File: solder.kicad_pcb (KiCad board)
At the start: 2 copper layers, 83.3 x 92.9 mm, 22 parts, among them M1 Motor_DC, SW2 SW_Push, SW3 SW_Push, SW4 SW_Push

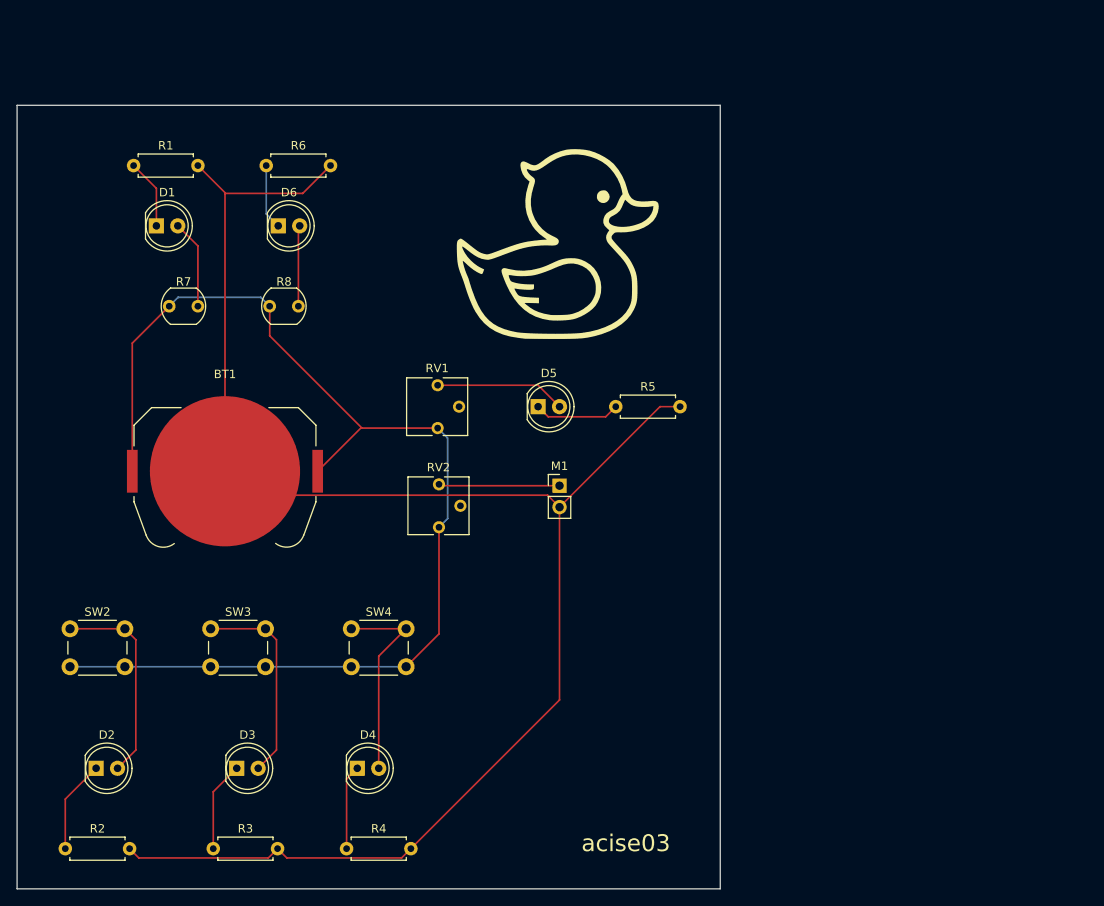
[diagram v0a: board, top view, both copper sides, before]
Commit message: gg
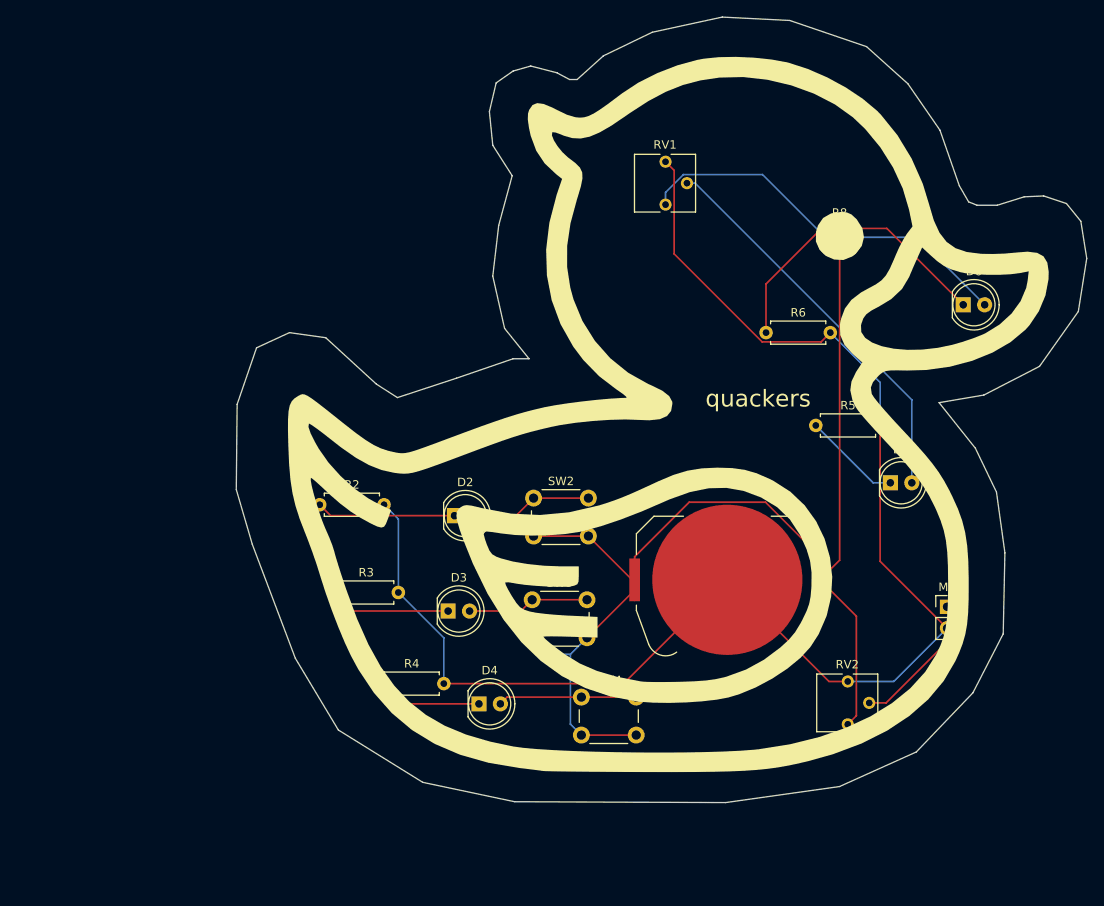
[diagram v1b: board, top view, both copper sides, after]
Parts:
- removed D1: LED, LED_THT:LED_D5.0mm
- removed R1: R, Resistor_THT:R_Axial_DIN0207_L6.3mm_D2.5mm_P7.62mm_Horizontal
- removed R7: R_Photo, OptoDevice:R_LDR_5.1x4.3mm_P3.4mm_Vertical
- moved D6 81.7 mm to (224.1, 54.6)
- moved R8 66.3 mm to (207.7, 46.6)
- moved R6 62.5 mm to (200.7, 57.9)
- moved BT1 60.9 mm to (196.1, 87.2)
- moved SW2 57.1 mm to (173.1, 77.5)
- moved RV2 53.8 mm to (210.4, 104.3)
- moved D2 52.0 mm to (163.8, 79.6)
- moved R2 50.7 mm to (147.8, 78.3)
- moved M1 48.1 mm to (222.1, 90.4)
- moved D5 42.7 mm to (215.4, 75.7)
- moved SW3 38.3 mm to (173.0, 89.6)
- moved RV1 37.8 mm to (188.8, 42.7)
- moved R3 33.6 mm to (149.5, 88.7)
- moved D3 31.2 mm to (163.0, 90.9)
- moved SW4 28.4 mm to (178.8, 101.1)
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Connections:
- RV1 pad 2: unconnected-(RV1-Pad2) -> Net-(D5-A)
- RV1 pad 3: Net-(D5-A) -> Net-(BT1--)
- RV2 pad 2: unconnected-(RV2-Pad2) -> Net-(M1-+)
- RV2 pad 3: Net-(M1-+) -> Net-(BT1--)
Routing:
- net Net-(BT1-+): track 140.1 -> 171.9 mm
- net Net-(D5-A): track 15.5 -> 47.1 mm
- net Net-(D6-K): track 7.74 -> 35.6 mm
- net Net-(BT1--): track 195.0 -> 172.2 mm
- net Net-(D1-A): track 10.5 -> 0.00 mm
- net Net-(D2-A): track 24.5 -> 14.2 mm
- net Net-(D3-A): track 24.5 -> 14.5 mm
- net Net-(D6-A): track 9.59 -> 18.8 mm
- net Net-(D1-K): track 8.26 -> 0.00 mm
- net Net-(D4-A): track 24.4 -> 16.4 mm
- net Net-(D2-K): track 11.0 -> 16.5 mm
- net Net-(D3-K): track 10.7 -> 14.4 mm
- net Net-(M1-+): track 14.4 -> 17.3 mm
- net Net-(D4-K): track 10.1 -> 12.8 mm
- net Net-(D5-K): track 10.2 -> 11.7 mm
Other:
- board size 83.3 x 92.9 mm -> 100.8 x 93.1 mm
- board text added: "quackers"
